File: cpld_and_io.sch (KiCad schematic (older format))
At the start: 3 parts, among them U11 5M1270ZT144C5N, U13 IS61LV5128AL-10TLI

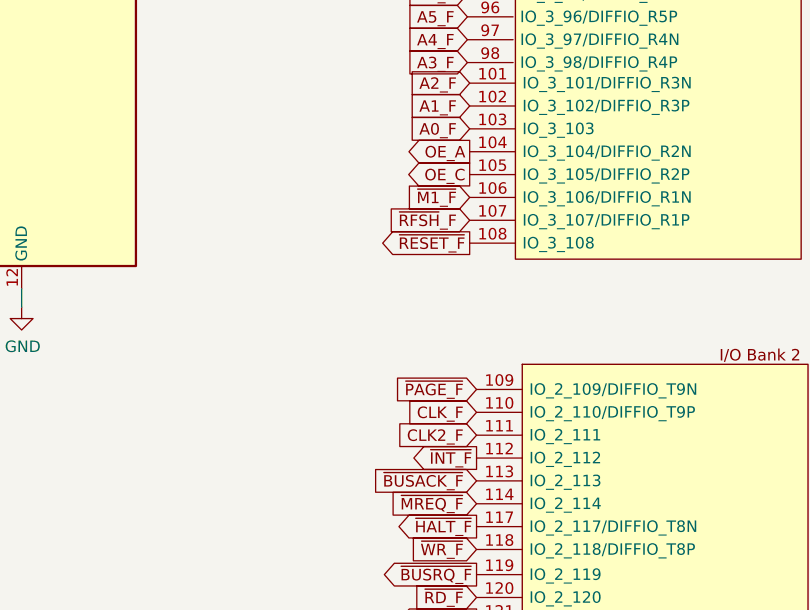
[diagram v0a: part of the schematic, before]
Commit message: started routing
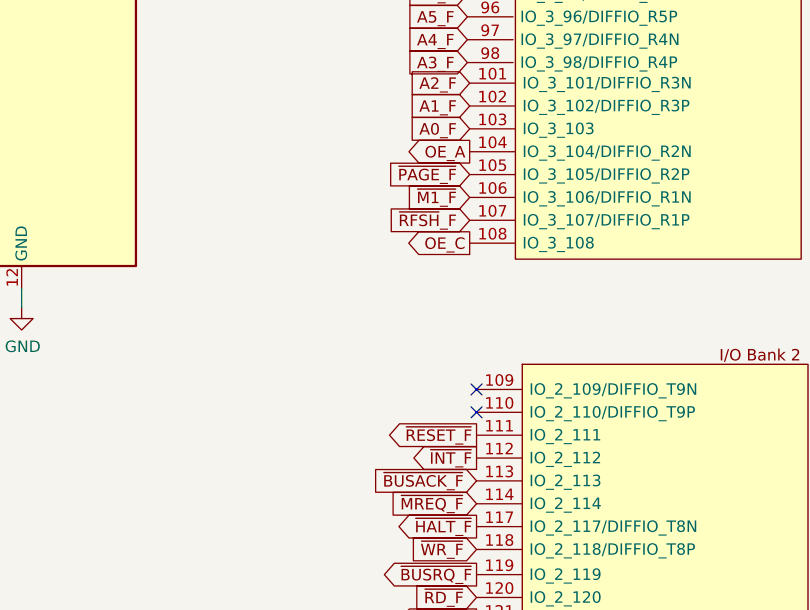
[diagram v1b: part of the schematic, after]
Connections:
- net CLK2_F is gone; now on net ~RESET_F: U11.111 (IO_2_111)
- net OE_C: now also U11.108 (IO_3_108); no longer U11.105 (IO_3_105/DIFFIO_R2P)
- net ~PAGE_F: now also U11.105 (IO_3_105/DIFFIO_R2P); no longer U11.109 (IO_2_109/DIFFIO_T9N)
- net ~RESET_F: no longer U11.108 (IO_3_108)
- net CLK_F: no longer names the net of U11.110 (IO_2_110/DIFFIO_T9P)
- no-connect marks 10 -> 12
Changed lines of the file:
@@
 Text GLabel 4420 4390 0    50   Input ~ 0
 ~BUSACK_F
-Text GLabel 4420 3990 0    50   Input ~ 0
+Text GLabel 4390 3050 0    50   Input ~ 0
 ~PAGE_F
 Text GLabel 4390 3150 0    50   Input ~ 0
 ~M1_F
-Text GLabel 4420 4090 0    50   Input ~ 0
-CLK_F
-Text GLabel 4390 3350 0    50   Output ~ 0
+Text GLabel 4420 4190 0    50   Output ~ 0
 ~RESET_F
 Text GLabel 4420 4290 0    50   Output ~ 0
@@
 Text GLabel 4390 3250 0    50   Input ~ 0
 ~RFSH~_F
-Text GLabel 4420 4190 0    50   Input ~ 0
-CLK2_F
 Text GLabel 4420 4490 0    50   Input ~ 0
 ~MREQ_F
@@
 Text GLabel 7020 1090 0    50   Input ~ 0
 RXA_F
-Text GLabel 7020 990  0    50   Output ~ 0
-TXA_F
-Text GLabel 7020 890  0    50   Input ~ 0
-RXB_F
 Text GLabel 7020 790  0    50   Output ~ 0
 TXB_F
@@
 Text GLabel 4390 2950 0    50   Output ~ 0
 OE_A
-Text GLabel 4390 3050 0    50   Output ~ 0
+Text GLabel 4390 3350 0    50   Output ~ 0
 OE_C
 Text GLabel 7040 4620 0    50   Output ~ 0
@@
 Text GLabel 7040 3330 0    50   BiDi ~ 0
 SCL
+Text GLabel 7020 890  0    50   Input ~ 0
+RXB_F
+Text GLabel 7020 990  0    50   Output ~ 0
+TXA_F
+NoConn ~ 4420 3990
+NoConn ~ 4420 4090
 $EndSCHEMATC
